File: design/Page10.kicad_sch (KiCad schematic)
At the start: 0 parts

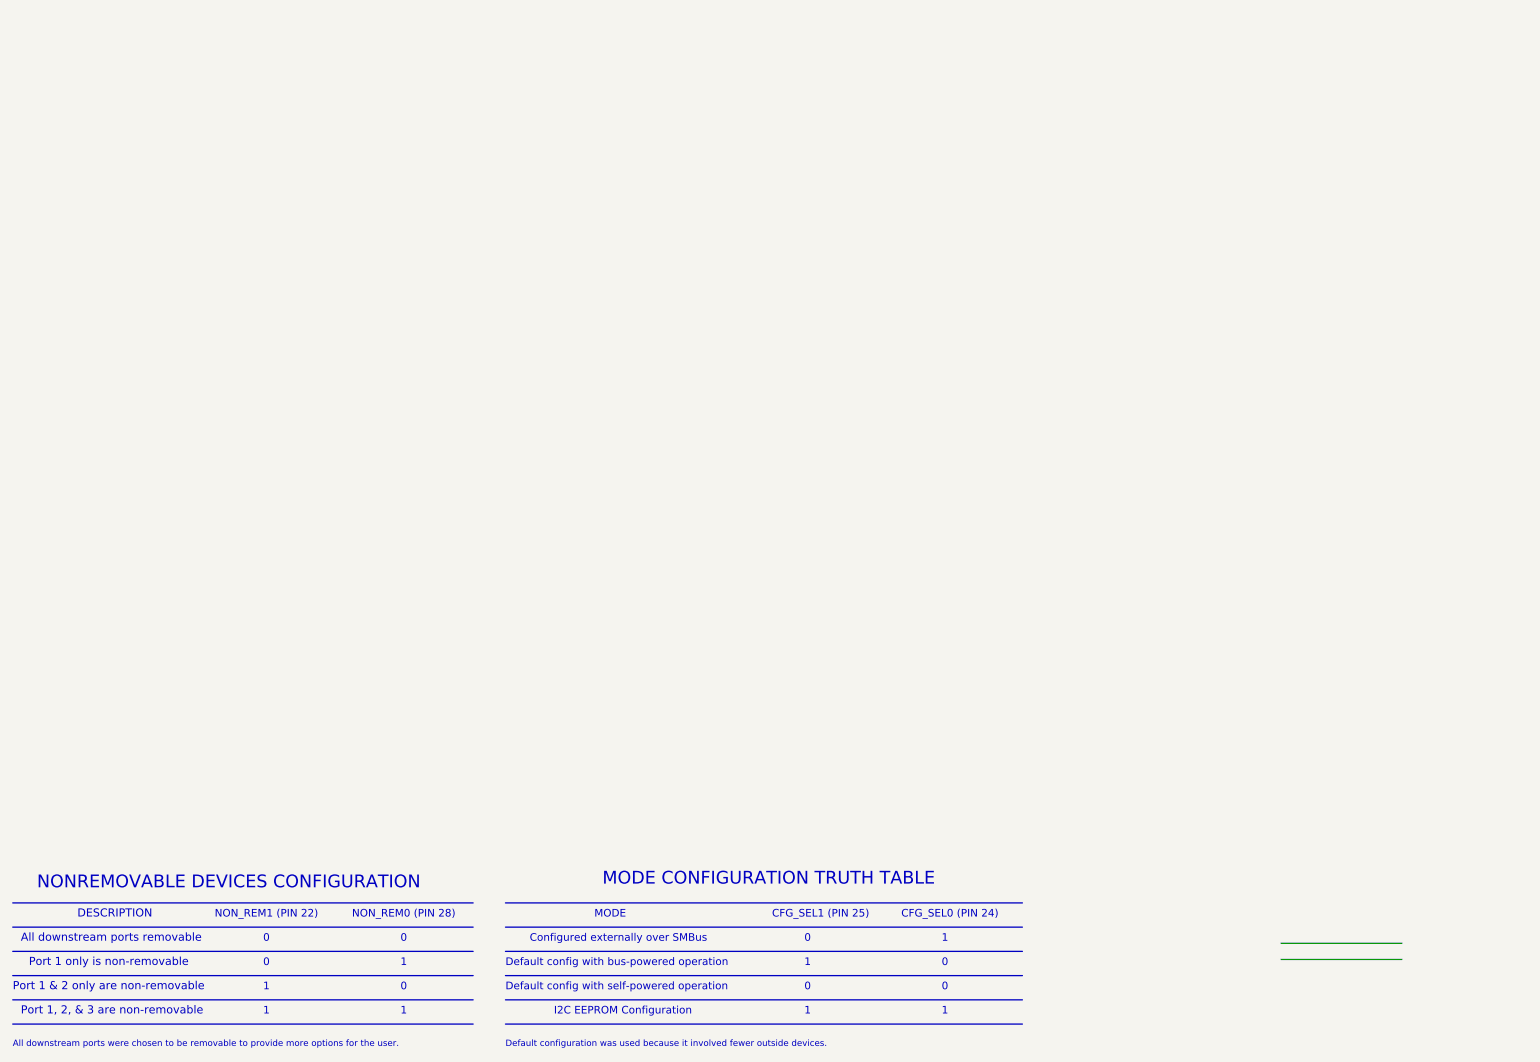
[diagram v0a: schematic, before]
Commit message: updated, its functional, but needs routing finished. tweeks from Bornhack 2026 to be added. :)
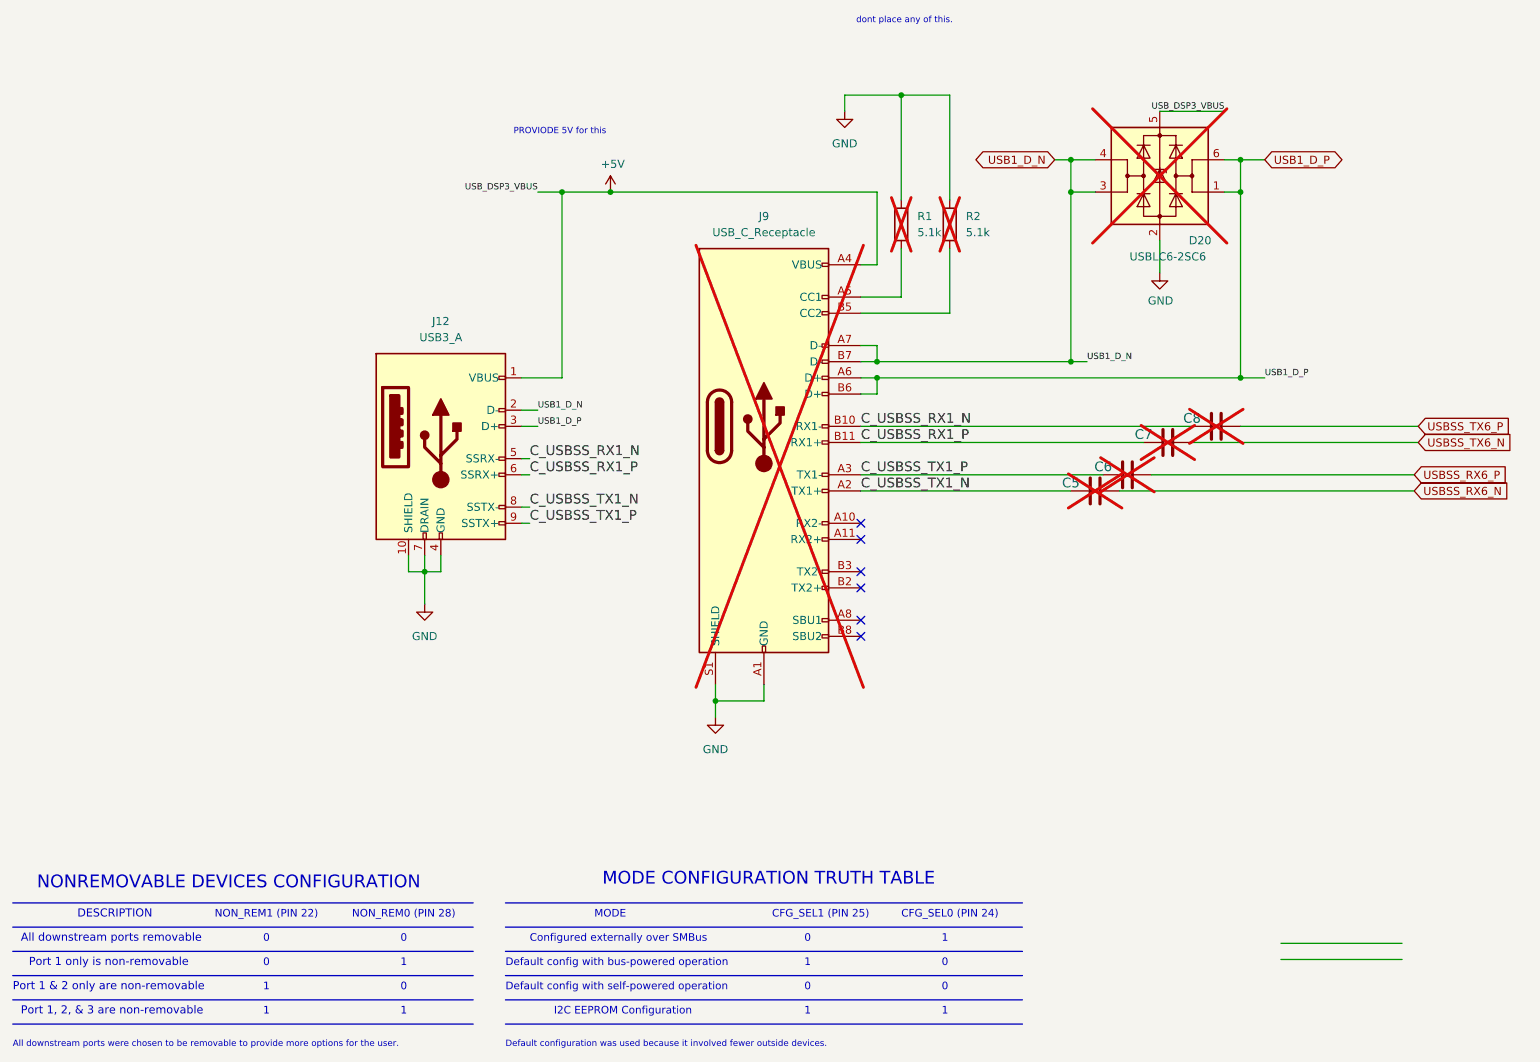
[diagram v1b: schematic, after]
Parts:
- added C5, C6, C7, C8: 0.1uF, Capacitor_SMD:C_0805_2012Metric_Pad1.18x1.45mm_HandSolder, symbol jetson-nano-baseboard:C_100n_0402
- added D20: USBLC6-2SC6, Package_TO_SOT_SMD:SOT-23-6, symbol Power_Protection:USBLC6-2SC6
- added J12: USB3_A, Connector_USB:USB3_A_Molex_48393-001, symbol Connector:USB3_A
- added J9: USB_C_Receptacle, Connector_USB:USB_C_Receptacle_Amphenol_12401548E4-2A, symbol Connector:USB_C_Receptacle
- added R1, R2: 5.1k, Resistor_SMD:R_0402_1005Metric, symbol Device:R
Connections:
- new net: J9.B5 (CC2), R2.2
- new net: J9.A5 (CC1), R1.2
- new net +5V: D20.5 (VBUS), J12.1 (VBUS), J9.A4 (VBUS), J9.A9 (VBUS), J9.B4 (VBUS), J9.B9 (VBUS)
- new net C_USBSS_RX1_N: C8.1, J12.5 (SSRX-), J9.B10 (RX1-)
- new net C_USBSS_RX1_P: C7.1, J12.6 (SSRX+), J9.B11 (RX1+)
- new net C_USBSS_TX1_N: C5.1, J12.8 (SSTX-), J9.A2 (TX1+)
- new net C_USBSS_TX1_P: C6.1, J12.9 (SSTX+), J9.A3 (TX1-)
- new net GND: D20.2 (GND), J12.10 (SHIELD), J12.4 (GND), J12.7 (DRAIN), J9.A1 (GND), J9.A12 (GND), J9.B1 (GND), J9.B12 (GND), J9.S1 (SHIELD), R1.1, R2.1
- new net USB1_D_N: D20.3 (I/O2), D20.4 (I/O2), J12.2 (D-), J9.A7 (D-), J9.B7 (D-)
- new net USB1_D_P: D20.1 (I/O1), D20.6 (I/O1), J12.3 (D+), J9.A6 (D+), J9.B6 (D+)
- new net USBSS_RX6_N: C5.2
- new net USBSS_RX6_P: C6.2
- new net USBSS_TX6_N: C7.2
- new net USBSS_TX6_P: C8.2
- no-connect marks 0 -> 6
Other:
- note added: "PROVIODE 5V for this"
- note added: "dont place any of this."

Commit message: cleaned up a bit, more to do
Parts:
- C5, C6, C7, C8: now in the parts list
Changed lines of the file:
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@@
 		(unit 1)
 		(exclude_from_sim no)
-		(in_bom no)
+		(in_bom yes)
 		(on_board yes)
 		(dnp yes)
@@
 		(unit 1)
 		(exclude_from_sim no)
-		(in_bom no)
+		(in_bom yes)
 		(on_board yes)
 		(dnp yes)
@@
 		(unit 1)
 		(exclude_from_sim no)
-		(in_bom no)
+		(in_bom yes)
 		(on_board yes)
 		(dnp yes)
@@
 		(unit 1)
 		(exclude_from_sim no)
-		(in_bom no)
+		(in_bom yes)
 		(on_board yes)
 		(dnp yes)
